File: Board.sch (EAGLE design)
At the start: 13 parts, among them IC1 317EMP, K1 G5LE, Q1 MOSFET-NCHANNELSMD

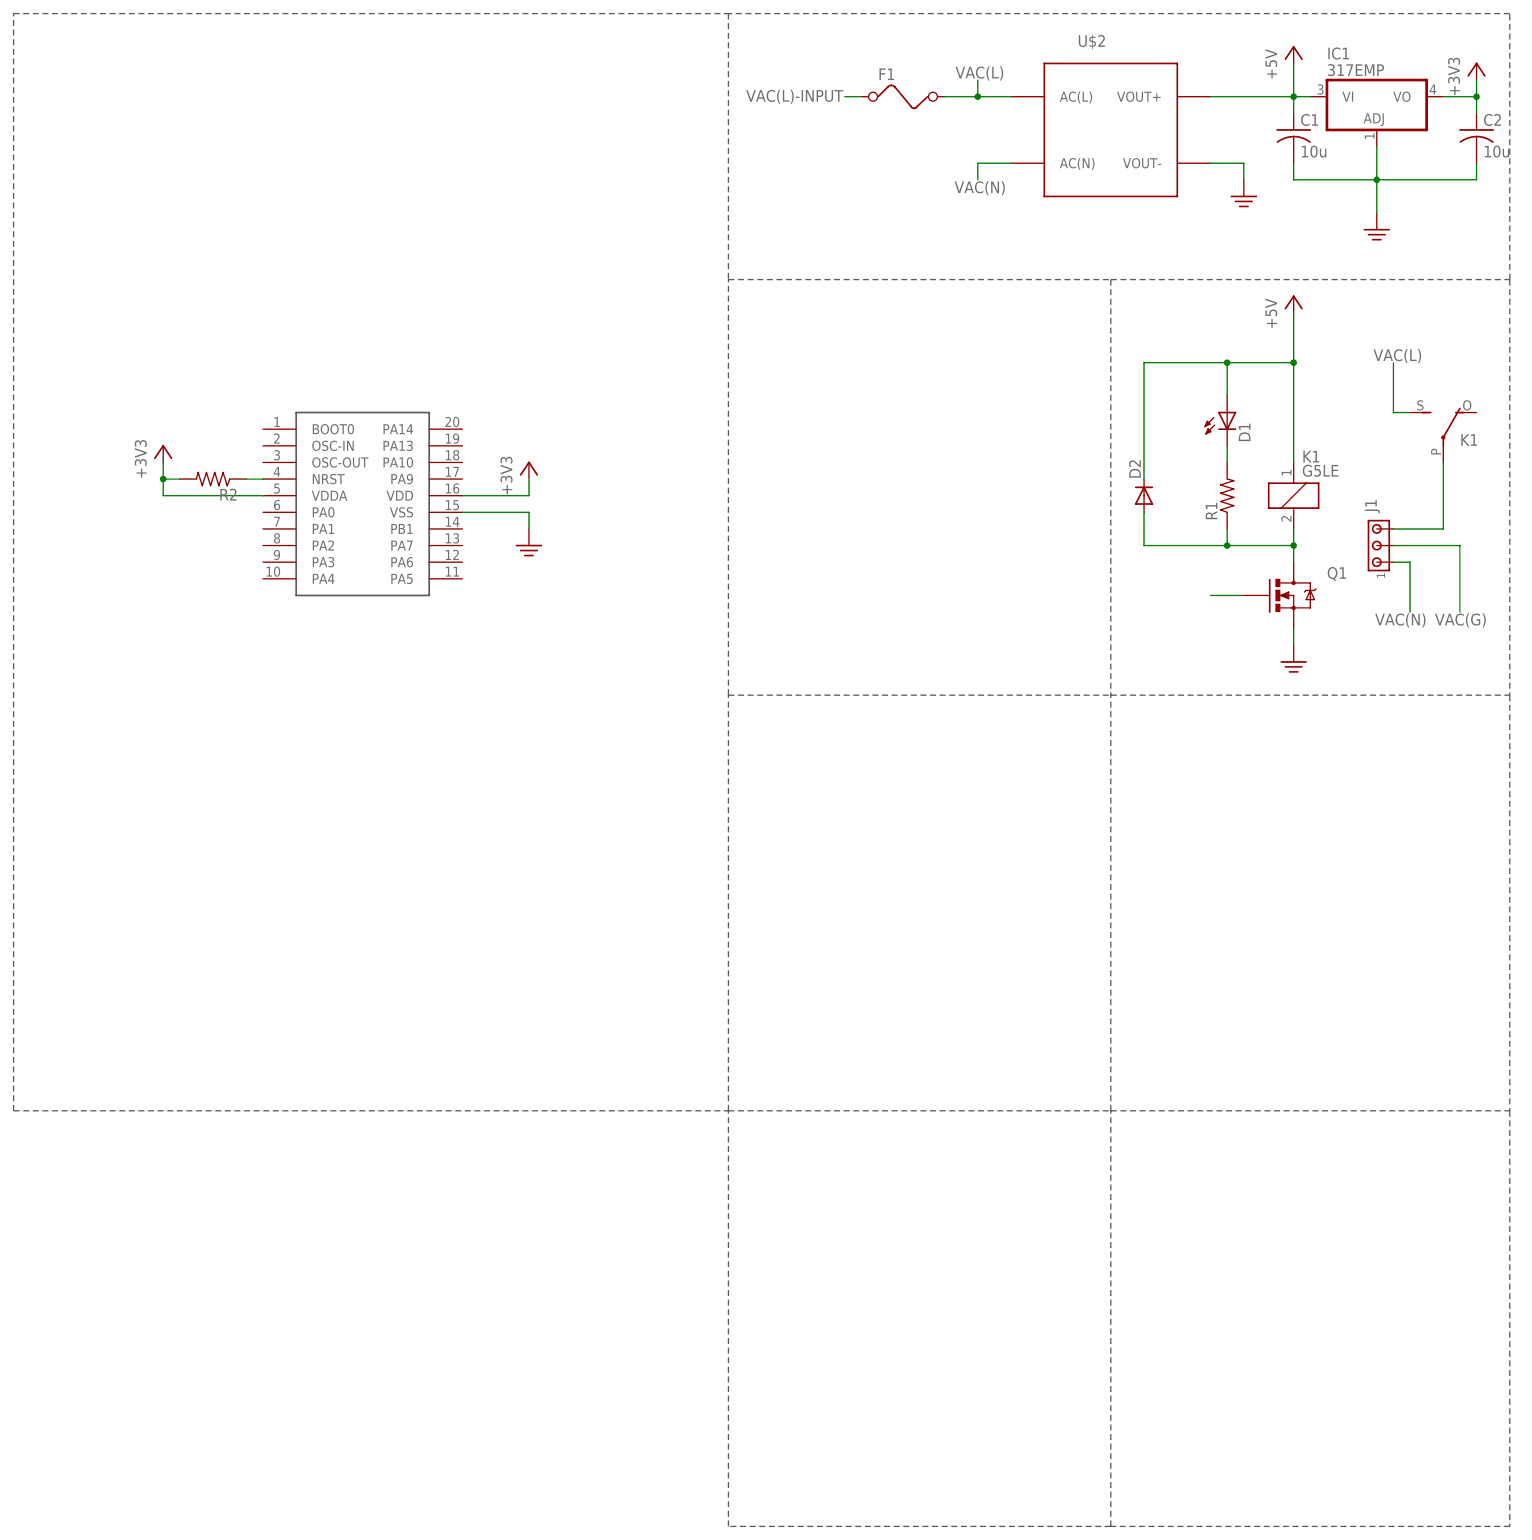
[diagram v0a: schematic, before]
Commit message: Worked on Schematic
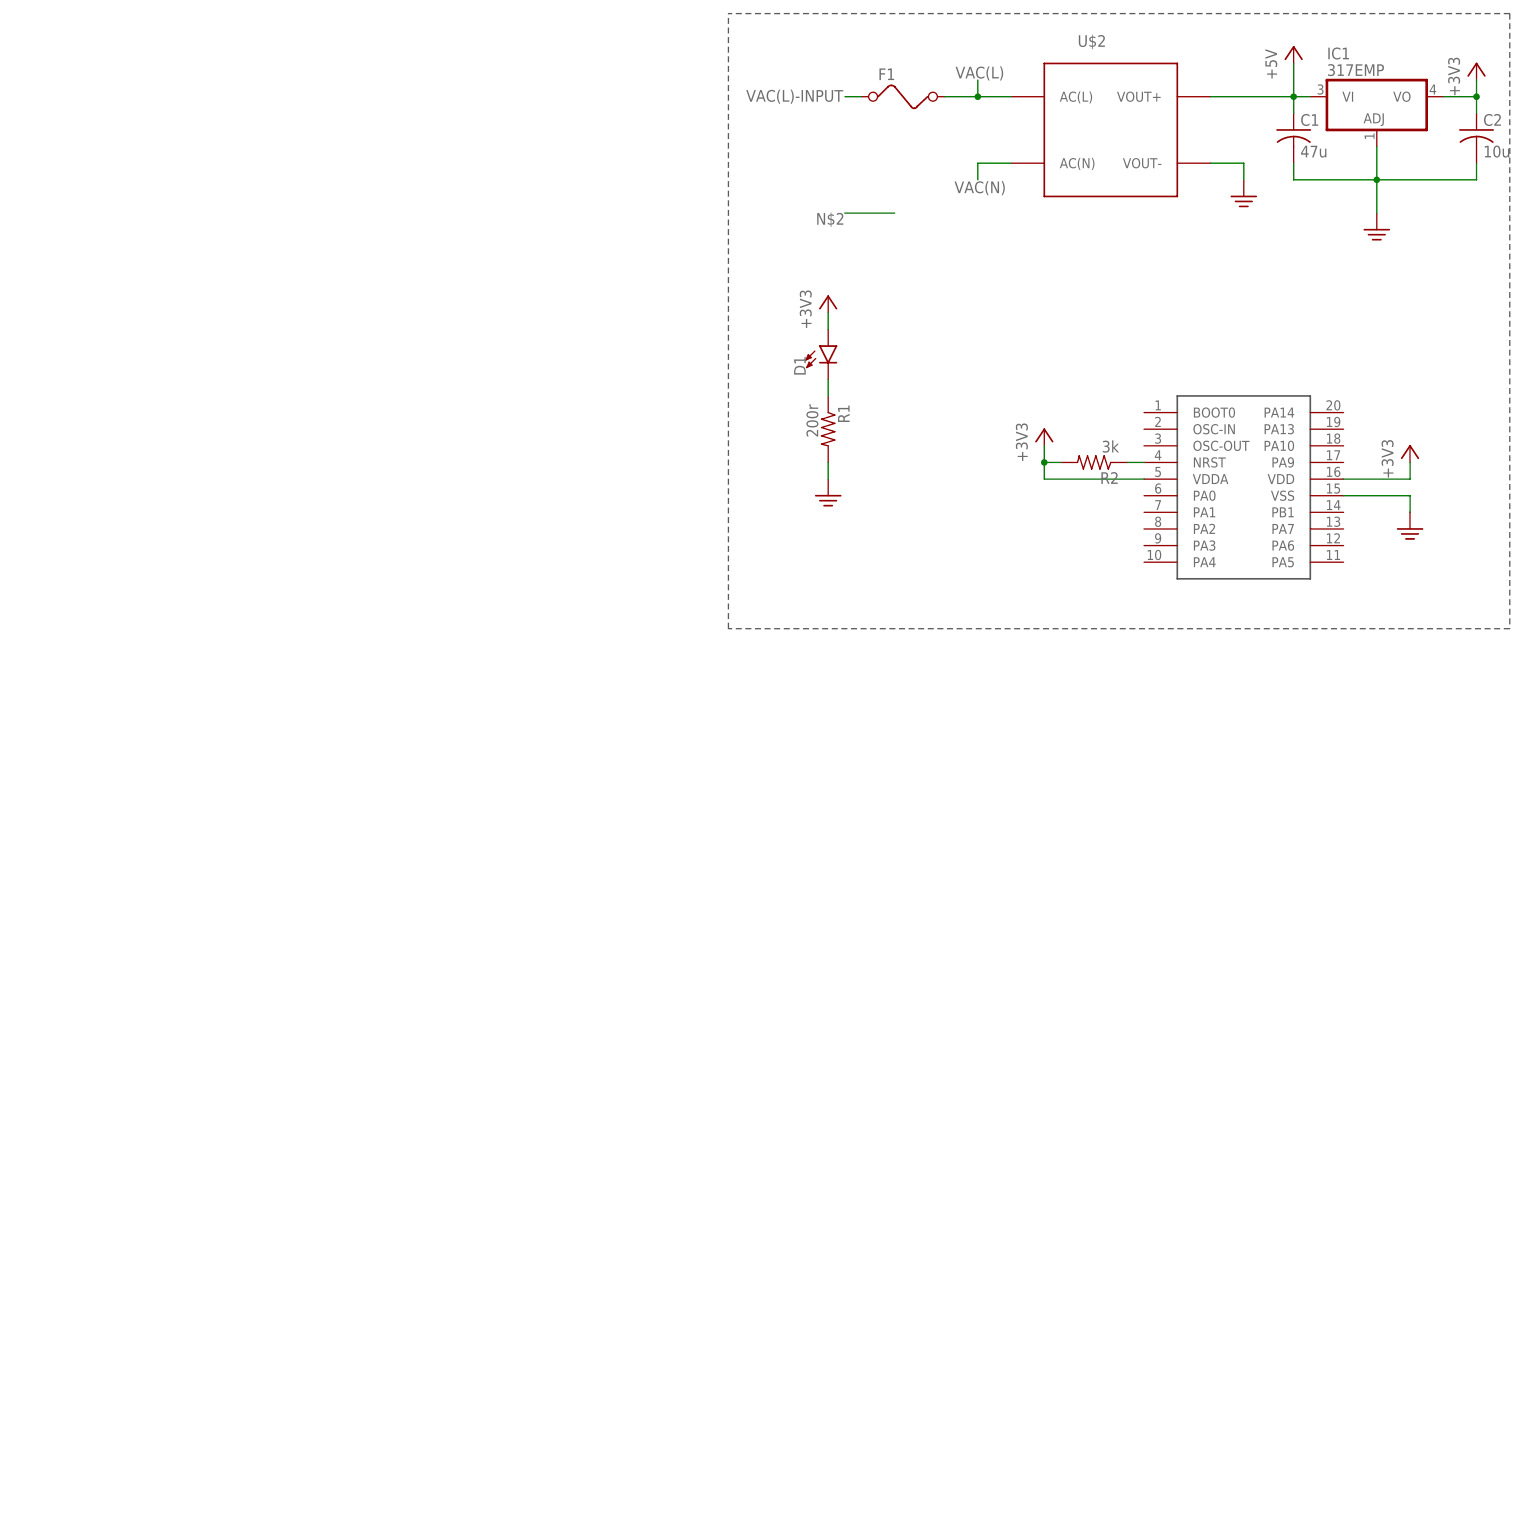
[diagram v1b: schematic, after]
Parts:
- removed D2: 1N4004, diode:1N4004
- removed J1: (no value), con-amp:MTA03-156
- removed K1: G5LE, relay:G5LE
- removed Q1: MOSFET-NCHANNELSMD, fets:MOSFET-NCHANNELSMD
- C1: value 10u -> 47u
- D1: value U57X32 -> GREEN; device led:U57X32 -> SparkFun-LED:LED-GREEN0603
- R1: value (none) -> 200r
- R2: value (none) -> 3k
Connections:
- removed net N$2: D1.C, R1.2
- removed net N$4: J1.3, K12.P
- removed net N$5: Q1.G
- removed net VAC(G): J1.2
- net +3V3: now also D1.A
- net +5V: no longer D1.A, D2.C, K11.1
- net N$1: now also D1.C; no longer D2.A, K11.2, Q1.D
- net PE: now also R1.2; no longer Q1.S
- net VAC(L): no longer K12.S
- net VAC(N): no longer J1.1
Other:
- moved on the sheet: R1, R2

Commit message: preliminary board design
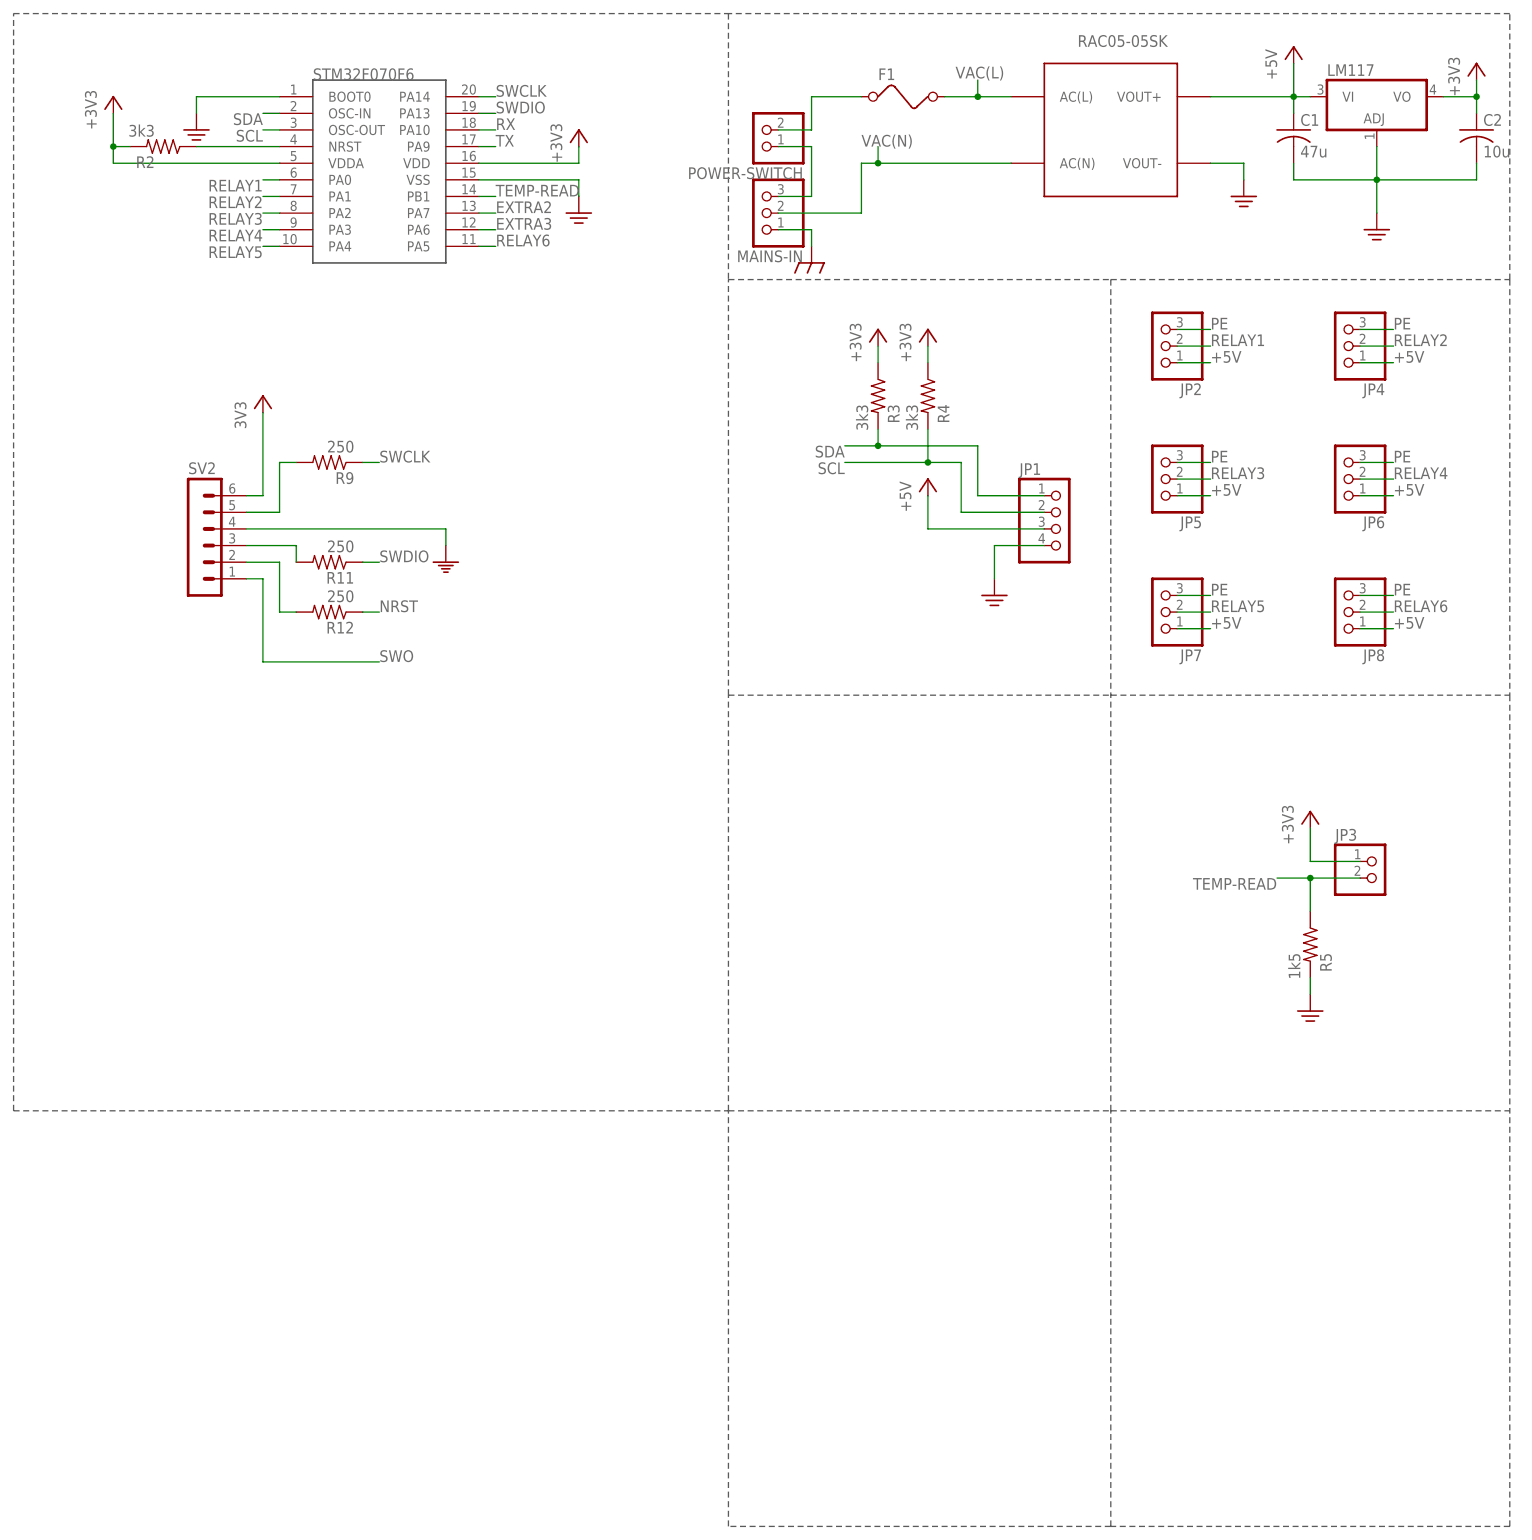
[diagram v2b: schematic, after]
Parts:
- removed D1: GREEN, SparkFun-LED:LED-GREEN0603
- removed R1: 200r, rcl:R-US_R0603
- removed U$1: STM32F07, chip:STM32F07
- added JP1: (no value), pinhead:PINHD-1X4
- added JP2, JP4, JP5, JP6, JP7, JP8, MAINS-IN: (no value), pinhead:PINHD-1X3
- added JP3, POWER-SWITCH: (no value), pinhead:PINHD-1X2
- added R11, R12, R9: 250, rcl:R-US_R0805
- added R3, R4: 3k3, rcl:R-US_R0603
- added R5: 1k5, rcl:R-US_R0603
- added STM32F070F6: STM32F07, SousVide Library:STM32F07
- added SV2: (no value), con-lstb:MA06-1
- R2: value 3k -> 3k3
- renumbered IC1 to LM117, U$2 to RAC05-05SK
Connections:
- removed net N$1: D1.C, R1.1
- removed net N$3: U$1.VDD
- removed net N$6: R2.1, U$1.NRST
- new net EXTRA2: STM32F070F6.PA7
- new net EXTRA3: STM32F070F6.PA6
- new net GND: SV2.4
- new net N$19: R9.2, SV2.5
- new net N$21: R11.2, SV2.3
- new net N$22: R12.2, SV2.2
- new net N$7: MAINS-IN.3, POWER-SWITCH.1
- new net NRST: R12.1, R2.1, STM32F070F6.NRST
- new net PGND: MAINS-IN.1
- new net RELAY1: JP2.2, STM32F070F6.PA0
- new net RELAY2: JP4.2, STM32F070F6.PA1
- new net RELAY3: JP5.2, STM32F070F6.PA2
- new net RELAY4: JP6.2, STM32F070F6.PA3
- new net RELAY5: JP7.2, STM32F070F6.PA4
- new net RELAY6: JP8.2, STM32F070F6.PA5
- new net RX: STM32F070F6.PA10
- new net SCL: JP1.2, R4.2, STM32F070F6.OSC-OUT
- new net SDA: JP1.1, R3.2, STM32F070F6.OSC-IN
- new net SWCLK: R9.1, STM32F070F6.PA14
- new net SWDIO: R11.1, STM32F070F6.PA13
- new net SWO: SV2.1
- new net TEMP-READ: JP3.2, R5.1, STM32F070F6.PB1
- new net TX: STM32F070F6.PA9
- net +3V3: now also JP3.1, R3.1, R4.1, STM32F070F6.VDD, STM32F070F6.VDDA, SV2.6; no longer D1.A, U$1.VDDA
- net +5V: now also JP1.3, JP2.1, JP4.1, JP5.1, JP6.1, JP7.1, JP8.1
- net PE: now also JP1.4, JP2.3, JP4.3, JP5.3, JP6.3, JP7.3, JP8.3, R5.2, STM32F070F6.BOOT0, STM32F070F6.VSS; no longer R1.2, U$1.VSS
- net VAC(L)-INPUT: now also POWER-SWITCH.2
- net VAC(N): now also MAINS-IN.2
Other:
- moved on the sheet: R2
